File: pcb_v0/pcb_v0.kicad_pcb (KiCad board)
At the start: 2 copper layers, 17 parts, among them J1 Screw_Terminal_01x03, U1 ATtiny2313-20P, U10 74141, U2 74141, U3 74141, U4 74141, U5 74LS377, U6 74141, U7 74141, U8 74LS377, U9 74LS377

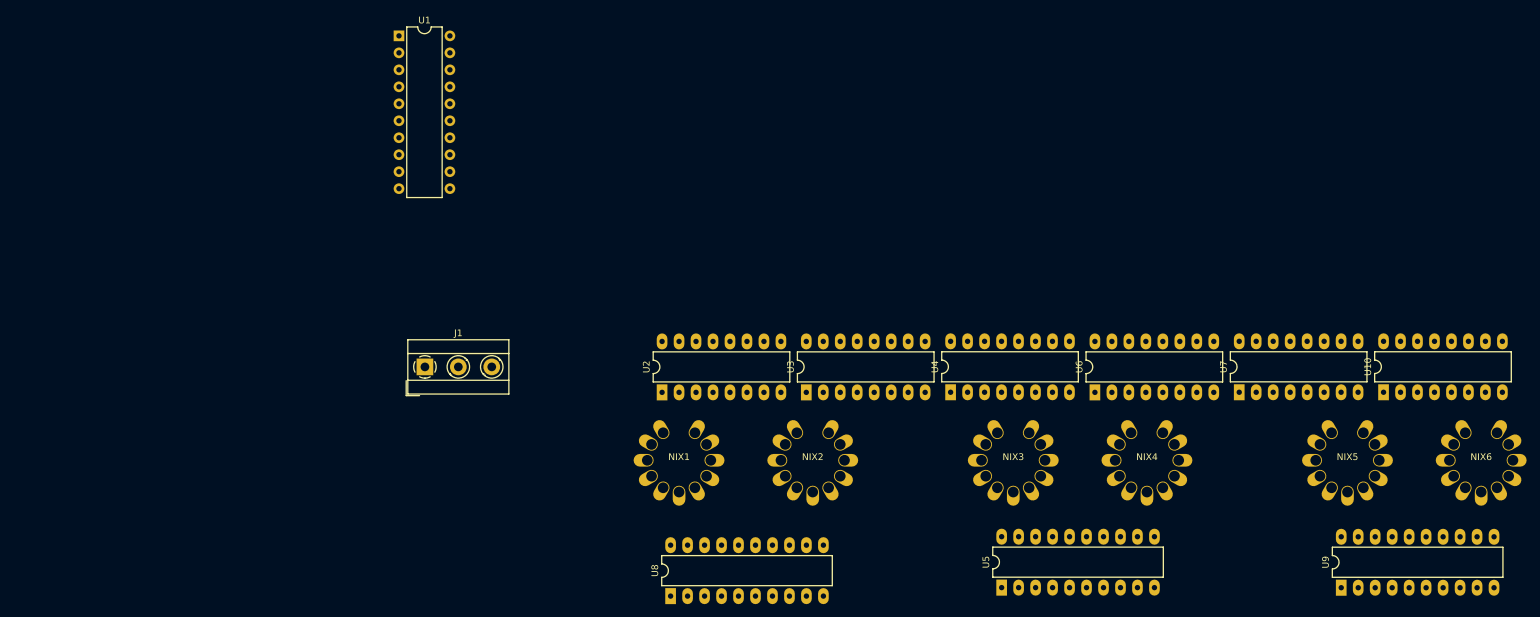
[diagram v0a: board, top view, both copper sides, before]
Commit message: saved
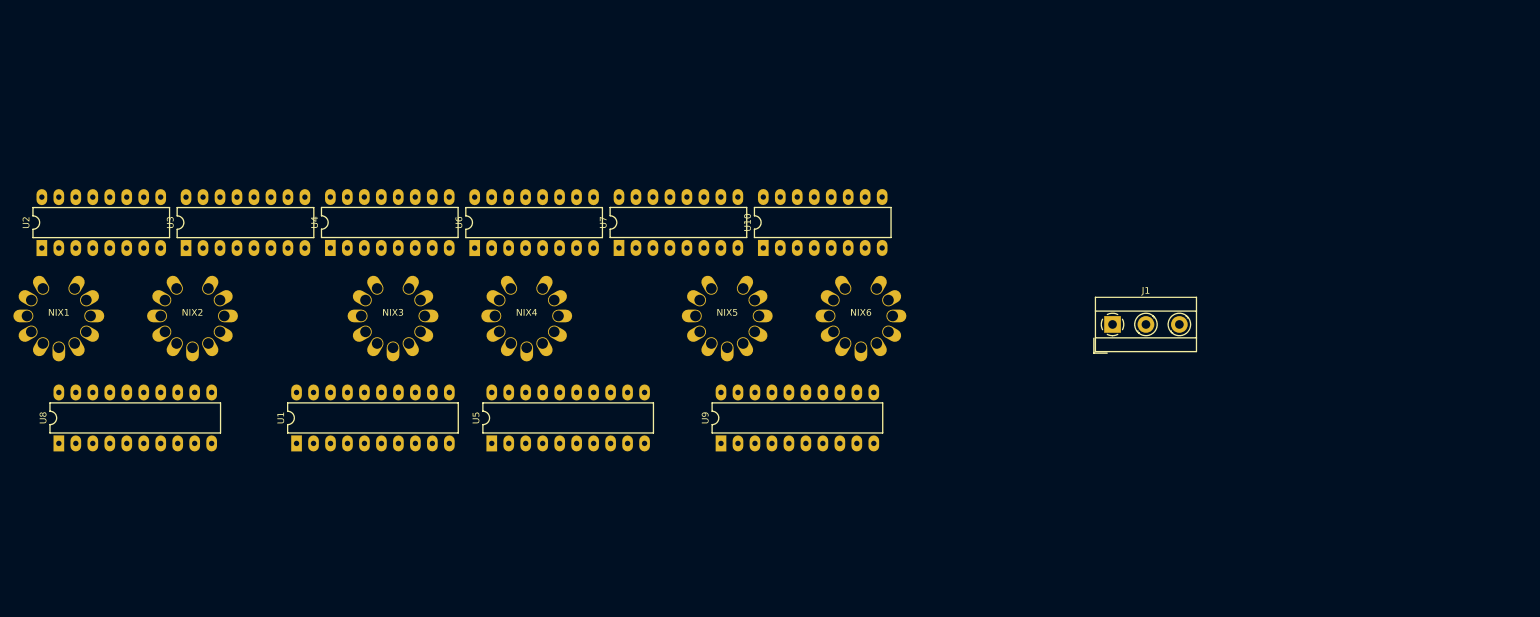
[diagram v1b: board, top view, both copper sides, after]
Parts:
- U1: footprint Package_DIP:DIP-20_W7.62mm -> Package_DIP:DIP-20_W7.62mm_LongPads
- moved J1 103.1 mm to (216.0, 61.0)
- moved U2 95.3 mm to (55.8, 49.5)
- moved NIX1 95.3 mm to (58.3, 59.7)
- moved NIX2 95.3 mm to (78.3, 59.7)
- moved NIX3 95.3 mm to (108.3, 59.7)
- moved NIX4 95.3 mm to (128.3, 59.7)
- moved NIX5 95.3 mm to (158.3, 59.7)
- moved NIX6 95.3 mm to (178.3, 59.7)
- moved U3 95.3 mm to (77.4, 49.5)
- moved U4 95.3 mm to (99.0, 49.5)
- moved U6 95.3 mm to (120.6, 49.5)
- moved U7 95.3 mm to (142.1, 49.5)
- moved U9 95.3 mm to (157.4, 78.8)
- moved U10 95.3 mm to (163.7, 49.5)
- moved U8 94.3 mm to (58.3, 78.8)
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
